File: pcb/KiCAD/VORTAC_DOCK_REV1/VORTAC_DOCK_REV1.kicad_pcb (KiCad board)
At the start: 4 copper layers, 25.4 x 16.4 mm, 26 parts, among them J1 Conn_01x05, J10 Conn_01x03, J7 Conn_01x01, J8 Conn_01x01, J9 Conn_01x03, U1 WS2811, U2 TPS26630RGE, U6 AP63205WU

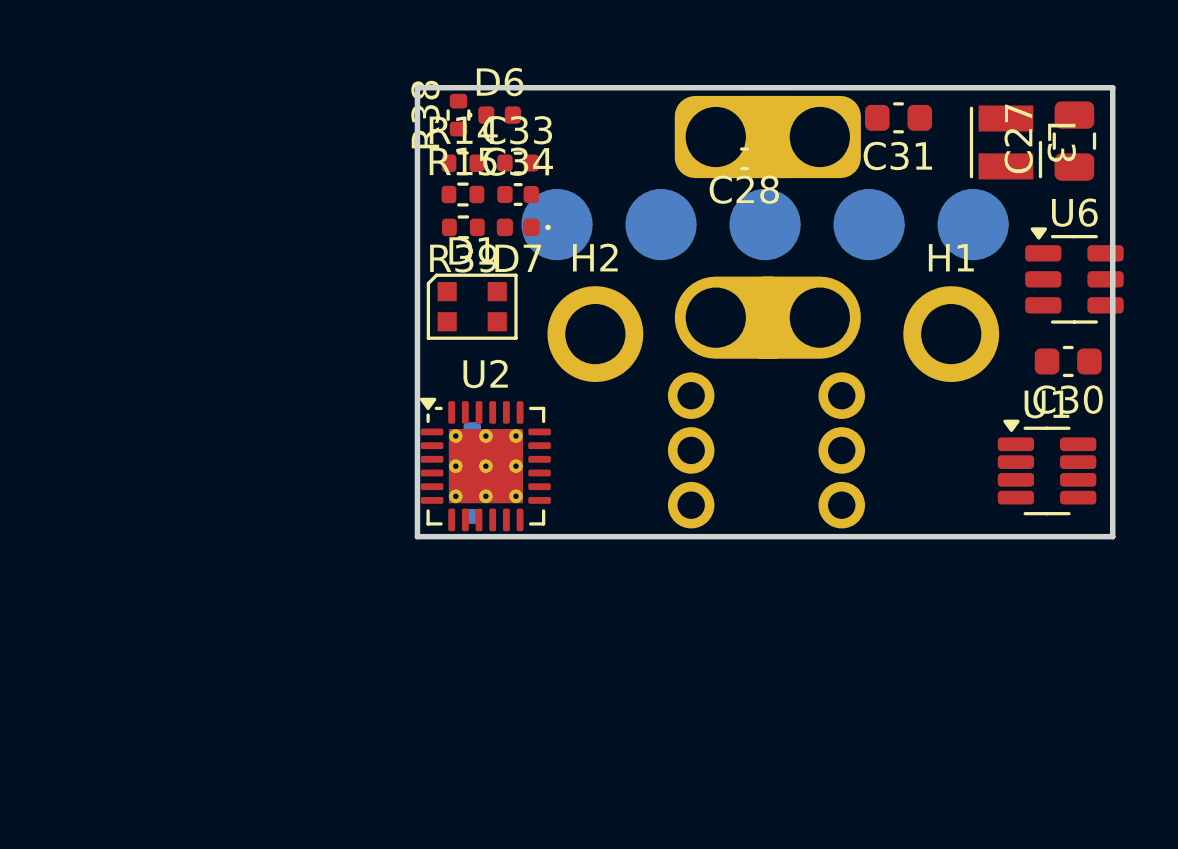
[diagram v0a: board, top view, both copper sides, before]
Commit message: Vortac Dock rough component placement #NO-JIRA
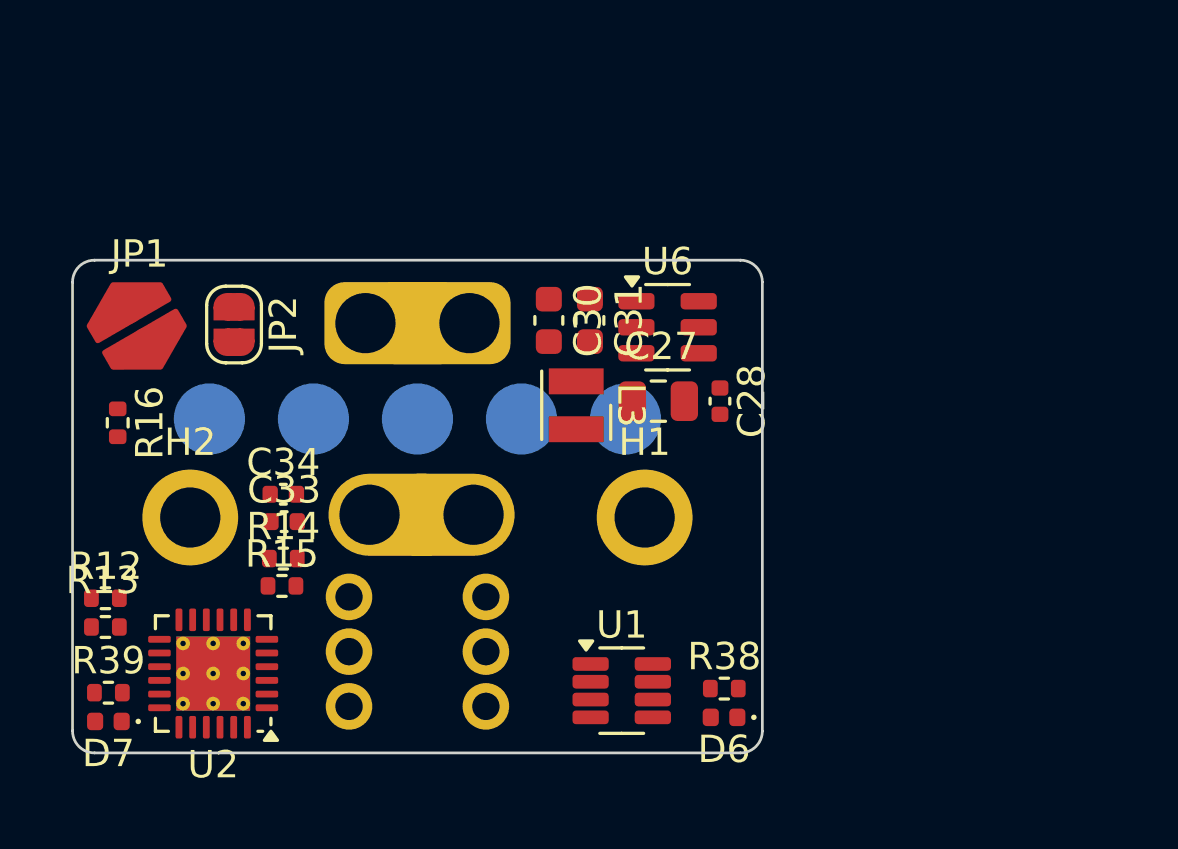
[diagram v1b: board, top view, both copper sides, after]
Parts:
- removed D1: NeoPixel_THT, LED_SMD:LED_WS2812B-2020_PLCC4_2.0x2.0mm
- added JP1: SolderJumper_2_Open, Vortac:SolderJumper_Hex_Open_Pad, F.Cu at (89.7, 106.7)
- added JP2: SolderJumper_2_Open, Jumper:SolderJumper-2_P1.3mm_Open_RoundedPad1.0x1.5mm, F.Cu at (93.3, 106.7)
- added R16: 120R, Resistor_SMD:R_0402_1005Metric, F.Cu at (89.0, 110.2)
- R12, R13: moved to F.Cu
- moved D6 23.5 mm to (111.2, 121.0), turned to 180 degrees
- moved D7 23.4 mm to (88.7, 121.2)
- moved R38 23.1 mm to (111.2, 120.0), turned to 0 degrees
- moved R39 21.4 mm to (88.7, 120.1), turned to 0 degrees
- moved C30 19.0 mm to (104.8, 106.5), turned to -90 degrees
- moved L3 18.4 mm to (105.8, 109.6)
- moved C27 17.9 mm to (108.8, 109.5), turned to 0 degrees
- moved U1 17.5 mm to (107.5, 120.0)
- moved H2 16.2 mm to (91.7, 113.7)
- moved R14 15.9 mm to (95.1, 115.2)
- moved R15 15.8 mm to (95.0, 116.2)
- moved C33 15.6 mm to (95.1, 113.8)
- moved R13 15.0 mm to (88.6, 117.7), turned to 0 degrees
- moved U6 15.0 mm to (109.1, 106.8)
- moved J10 14.9 mm to (102.5, 116.6)
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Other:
- board size 25.4 x 16.4 mm -> 25.2 x 18 mm
